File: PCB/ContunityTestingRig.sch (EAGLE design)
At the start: 29 parts

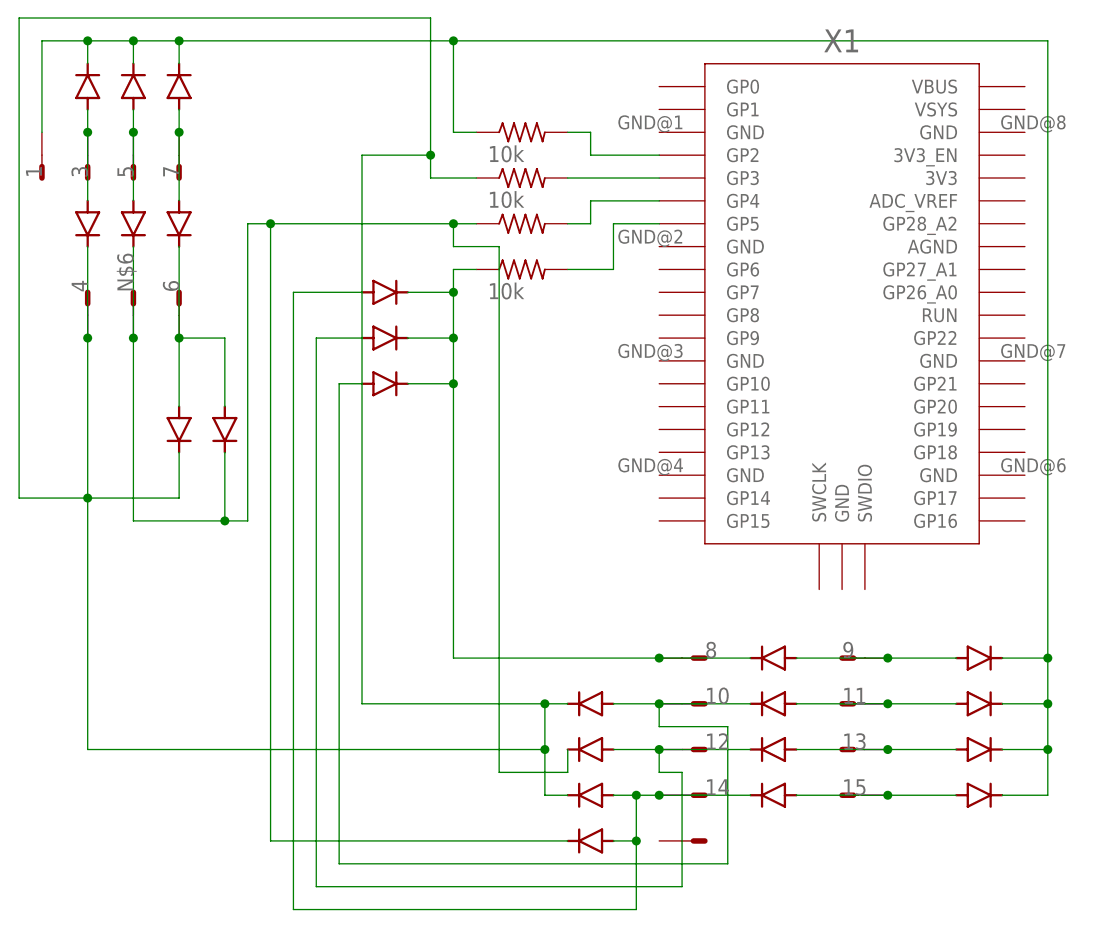
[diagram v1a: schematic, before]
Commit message: Updates
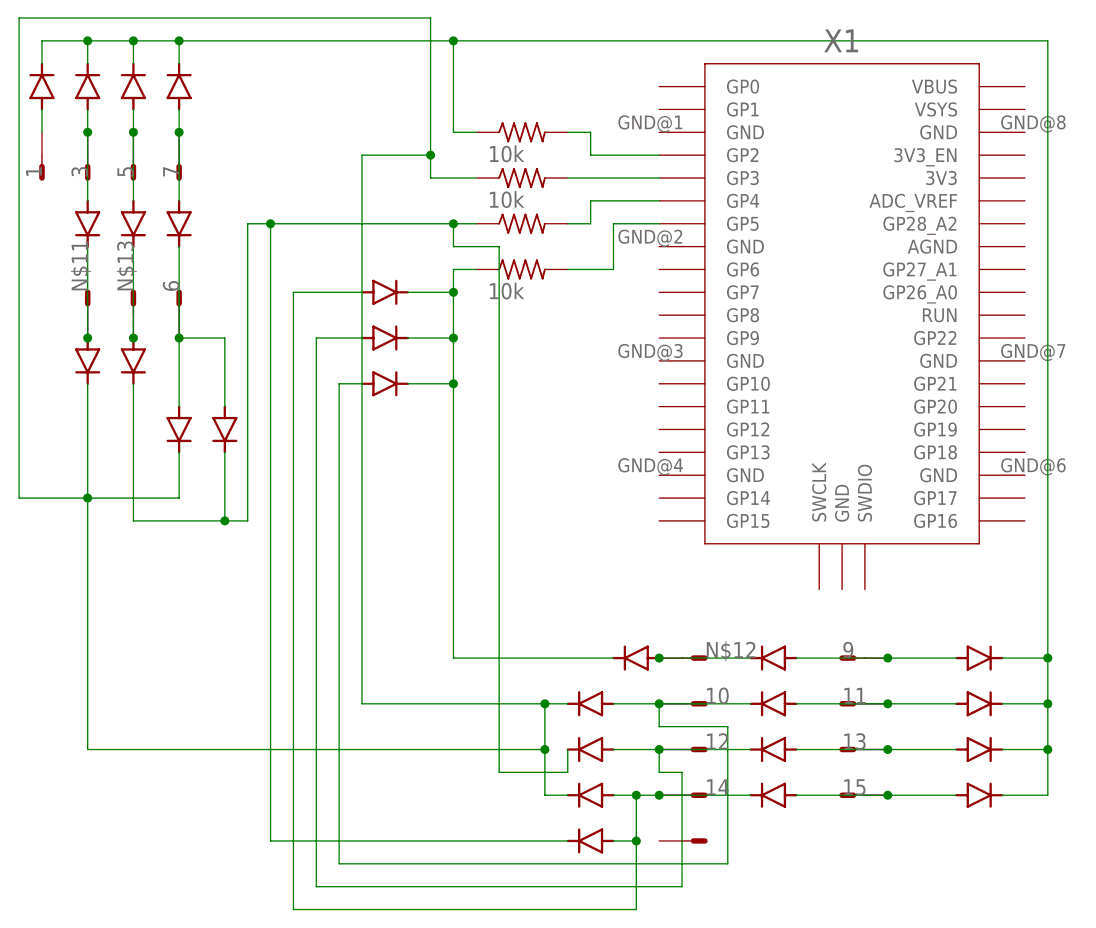
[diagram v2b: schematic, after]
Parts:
- added D24, D25, D26, D27: SCHOTTKY, eagle_fab:DIODE_SCHOTTKY_CDBM1100-G
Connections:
- new net N$10: D24.ANODE, SV1-1.S
- new net N$11: D25.ANODE, D4.KATHODE, SV1-2.S
- new net N$12: D26.ANODE, D9.KATHODE, SV1-8.S
- new net N$13: D27.ANODE, D5.KATHODE, SV1-4.S
- net 1: now also D24.KATHODE; no longer SV1-1.S
- net 4: now also D25.KATHODE; no longer D4.KATHODE, SV1-2.S
- net 8: now also D26.KATHODE; no longer D9.KATHODE, SV1-8.S
- net N$6: now also D27.KATHODE; no longer D5.KATHODE, SV1-4.S
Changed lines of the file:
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@@
 <part name="D22" library="eagle_fab" deviceset="DIODE_SCHOTTKY_CDBM1100-G" device="" value="SCHOTTKY"/>
 <part name="D23" library="eagle_fab" deviceset="DIODE_SCHOTTKY_CDBM1100-G" device="" value="SCHOTTKY"/>
+<part name="D24" library="eagle_fab" deviceset="DIODE_SCHOTTKY_CDBM1100-G" device="" value="SCHOTTKY"/>
+<part name="D25" library="eagle_fab" deviceset="DIODE_SCHOTTKY_CDBM1100-G" device="" value="SCHOTTKY"/>
+<part name="D26" library="eagle_fab" deviceset="DIODE_SCHOTTKY_CDBM1100-G" device="" value="SCHOTTKY"/>
+<part name="D27" library="eagle_fab" deviceset="DIODE_SCHOTTKY_CDBM1100-G" device="" value="SCHOTTKY"/>
 </parts>
 <sheets>
@@
 <instance part="D22" gate="G$1" x="35.56" y="27.94" smashed="yes" rot="R180"/>
 <instance part="D23" gate="G$1" x="35.56" y="22.86" smashed="yes" rot="R180"/>
+<instance part="D24" gate="G$1" x="-2.54" y="55.88" smashed="yes" rot="R270"/>
+<instance part="D25" gate="G$1" x="2.54" y="25.4" smashed="yes" rot="R90"/>
+<instance part="D26" gate="G$1" x="63.5" y="-7.62" smashed="yes"/>
+<instance part="D27" gate="G$1" x="7.62" y="25.4" smashed="yes" rot="R90"/>
 </instances>
 <busses>
@@
 <net name="8" class="0">
 <segment>
-<pinref part="D9" gate="G$1" pin="KATHODE"/>
-<pinref part="SV1" gate="-8" pin="S"/>
-<wire x1="76.2" y1="-7.62" x2="66.04" y2="-7.62" width="0.1524" layer="91"/>
 <pinref part="R4" gate="G$1" pin="1"/>
 <wire x1="43.18" y1="35.56" x2="45.72" y2="35.56" width="0.1524" layer="91"/>
-<wire x1="66.04" y1="-7.62" x2="43.18" y2="-7.62" width="0.1524" layer="91"/>
 <wire x1="43.18" y1="-7.62" x2="43.18" y2="22.86" width="0.1524" layer="91"/>
-<junction x="66.04" y="-7.62"/>
 <pinref part="D21" gate="G$1" pin="KATHODE"/>
 <wire x1="43.18" y1="22.86" x2="43.18" y2="27.94" width="0.1524" layer="91"/>
@@
 <wire x1="38.1" y1="22.86" x2="43.18" y2="22.86" width="0.1524" layer="91"/>
 <junction x="43.18" y="22.86"/>
-<label x="71.12" y="-7.62" size="1.778" layer="95"/>
+<pinref part="D26" gate="G$1" pin="KATHODE"/>
+<wire x1="60.96" y1="-7.62" x2="43.18" y2="-7.62" width="0.1524" layer="91"/>
 </segment>
 </net>
@@
 <net name="1" class="0">
 <segment>
-<pinref part="SV1" gate="-1" pin="S"/>
-<wire x1="-2.54" y1="50.8" x2="-2.54" y2="60.96" width="0.1524" layer="91"/>
 <pinref part="D1" gate="G$1" pin="KATHODE"/>
 <wire x1="-2.54" y1="60.96" x2="2.54" y2="60.96" width="0.1524" layer="91"/>
@@
 <junction x="109.22" y="-7.62"/>
 <label x="-2.54" y="45.72" size="1.778" layer="95" rot="R90"/>
+<pinref part="D24" gate="G$1" pin="KATHODE"/>
+<wire x1="-2.54" y1="58.42" x2="-2.54" y2="60.96" width="0.1524" layer="91"/>
 </segment>
 </net>
 <net name="4" class="0">
 <segment>
-<pinref part="D4" gate="G$1" pin="KATHODE"/>
-<pinref part="SV1" gate="-2" pin="S"/>
-<wire x1="2.54" y1="38.1" x2="2.54" y2="27.94" width="0.1524" layer="91"/>
-<wire x1="2.54" y1="27.94" x2="2.54" y2="10.16" width="0.1524" layer="91"/>
-<junction x="2.54" y="27.94"/>
 <pinref part="D7" gate="G$1" pin="KATHODE"/>
 <wire x1="2.54" y1="10.16" x2="12.7" y2="10.16" width="0.1524" layer="91"/>
@@
 <wire x1="-5.08" y1="10.16" x2="2.54" y2="10.16" width="0.1524" layer="91"/>
 <junction x="2.54" y="10.16"/>
-<label x="2.54" y="33.02" size="1.778" layer="95" rot="R90"/>
 <wire x1="2.54" y1="10.16" x2="2.54" y2="-17.78" width="0.1524" layer="91"/>
 <pinref part="D17" gate="G$1" pin="KATHODE"/>
@@
 <wire x1="2.54" y1="-17.78" x2="53.34" y2="-17.78" width="0.1524" layer="91"/>
 <junction x="53.34" y="-17.78"/>
+<pinref part="D25" gate="G$1" pin="KATHODE"/>
+<wire x1="2.54" y1="22.86" x2="2.54" y2="10.16" width="0.1524" layer="91"/>
 </segment>
 </net>
@@
 <pinref part="R3" gate="G$1" pin="1"/>
 <wire x1="22.86" y1="40.64" x2="43.18" y2="40.64" width="0.1524" layer="91"/>
-<pinref part="SV1" gate="-4" pin="S"/>
-<pinref part="D5" gate="G$1" pin="KATHODE"/>
 <wire x1="43.18" y1="40.64" x2="45.72" y2="40.64" width="0.1524" layer="91"/>
-<wire x1="7.62" y1="38.1" x2="7.62" y2="27.94" width="0.1524" layer="91"/>
-<junction x="7.62" y="27.94"/>
-<wire x1="7.62" y1="7.62" x2="7.62" y2="27.94" width="0.1524" layer="91"/>
 <pinref part="D8" gate="G$1" pin="KATHODE"/>
 <wire x1="17.78" y1="15.24" x2="17.78" y2="7.62" width="0.1524" layer="91"/>
@@
 <pinref part="D20" gate="G$1" pin="KATHODE"/>
 <wire x1="55.88" y1="-27.94" x2="22.86" y2="-27.94" width="0.1524" layer="91"/>
-<label x="7.62" y="33.02" size="1.778" layer="95" rot="R90"/>
 <wire x1="43.18" y1="38.1" x2="43.18" y2="40.64" width="0.1524" layer="91"/>
 <junction x="43.18" y="40.64"/>
-</segment>
-</net>
+<pinref part="D27" gate="G$1" pin="KATHODE"/>
+<wire x1="7.62" y1="22.86" x2="7.62" y2="7.62" width="0.1524" layer="91"/>
+</segment>
+</net>
+<net name="N$10" class="0">
+<segment>
+<pinref part="D24" gate="G$1" pin="ANODE"/>
+<pinref part="SV1" gate="-1" pin="S"/>
+<wire x1="-2.54" y1="53.34" x2="-2.54" y2="50.8" width="0.1524" layer="91"/>
+</segment>
+</net>
+<net name="N$11" class="0">
+<segment>
+<pinref part="SV1" gate="-2" pin="S"/>
+<pinref part="D4" gate="G$1" pin="KATHODE"/>
+<wire x1="2.54" y1="38.1" x2="2.54" y2="27.94" width="0.1524" layer="91"/>
+<label x="2.54" y="33.02" size="1.778" layer="95" rot="R90"/>
+<pinref part="D25" gate="G$1" pin="ANODE"/>
+<junction x="2.54" y="27.94"/>
+</segment>
+</net>
+<net name="N$12" class="0">
+<segment>
+<pinref part="SV1" gate="-8" pin="S"/>
+<pinref part="D9" gate="G$1" pin="KATHODE"/>
+<wire x1="76.2" y1="-7.62" x2="66.04" y2="-7.62" width="0.1524" layer="91"/>
+<label x="71.12" y="-7.62" size="1.778" layer="95"/>
+<pinref part="D26" gate="G$1" pin="ANODE"/>
+<junction x="66.04" y="-7.62"/>
+</segment>
+</net>
+<net name="N$13" class="0">
+<segment>
+<pinref part="SV1" gate="-4" pin="S"/>
+<pinref part="D5" gate="G$1" pin="KATHODE"/>
+<wire x1="7.62" y1="38.1" x2="7.62" y2="27.94" width="0.1524" layer="91"/>
+<label x="7.62" y="33.02" size="1.778" layer="95" rot="R90"/>
+<pinref part="D27" gate="G$1" pin="ANODE"/>
+<junction x="7.62" y="27.94"/>
+</segment>
+</net>
